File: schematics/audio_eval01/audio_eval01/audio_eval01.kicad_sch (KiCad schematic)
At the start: 21 parts, among them J1 Conn_01x10_Pin, J2 AudioJack3, J3 Conn_01x02_Pin, U2 AMS1117-1.8

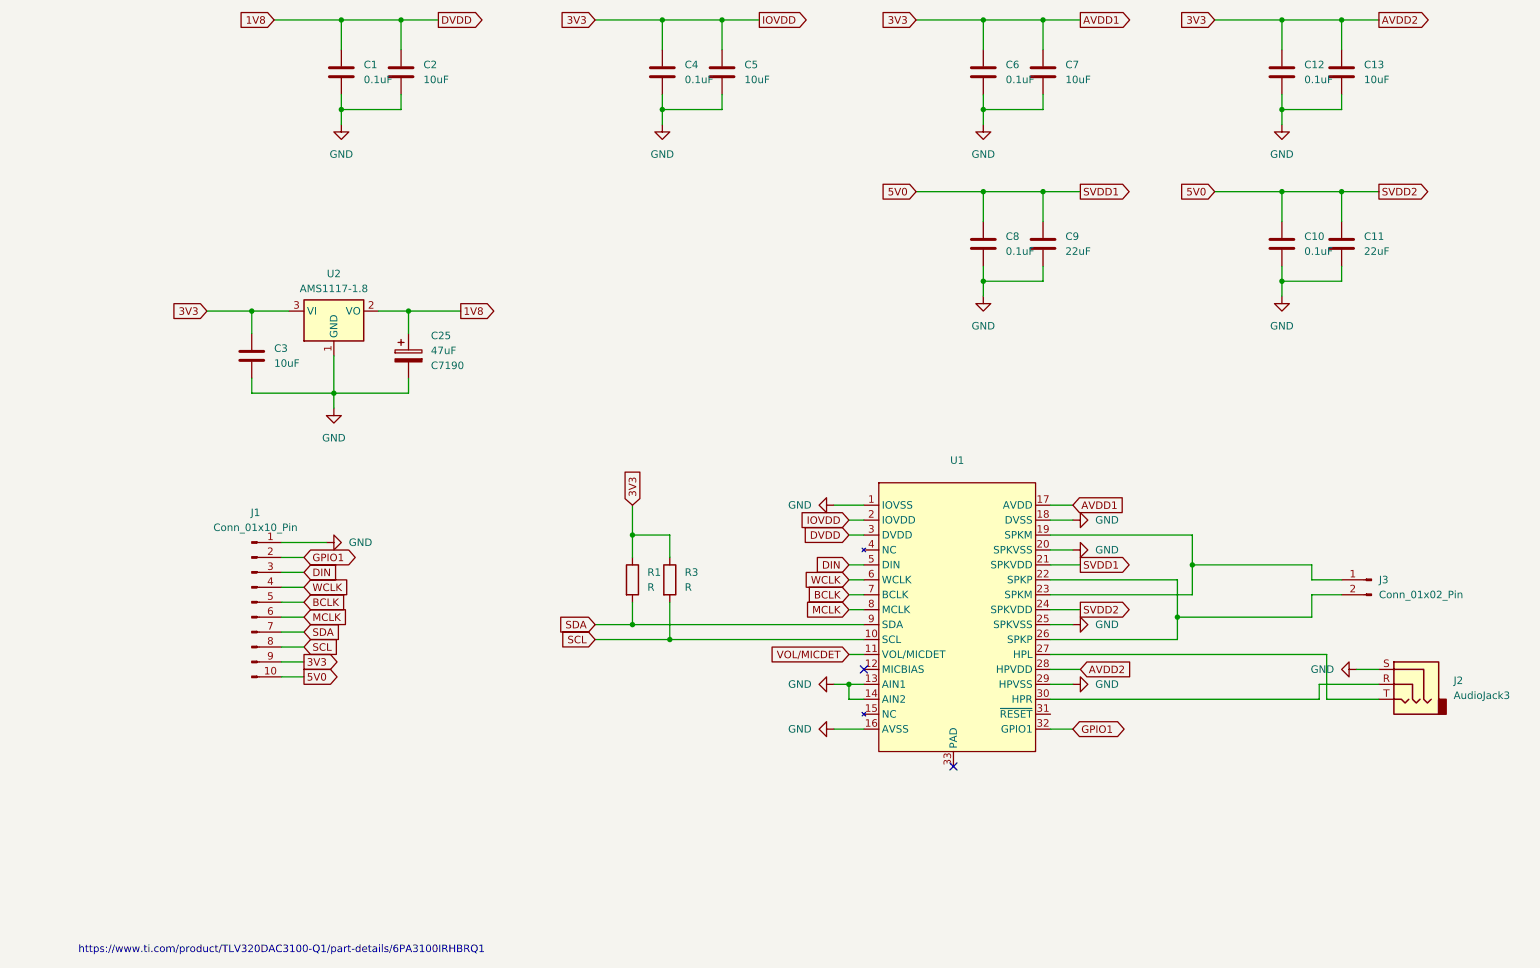
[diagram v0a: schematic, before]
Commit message: Prepared Audio evaluation board for manufacture.
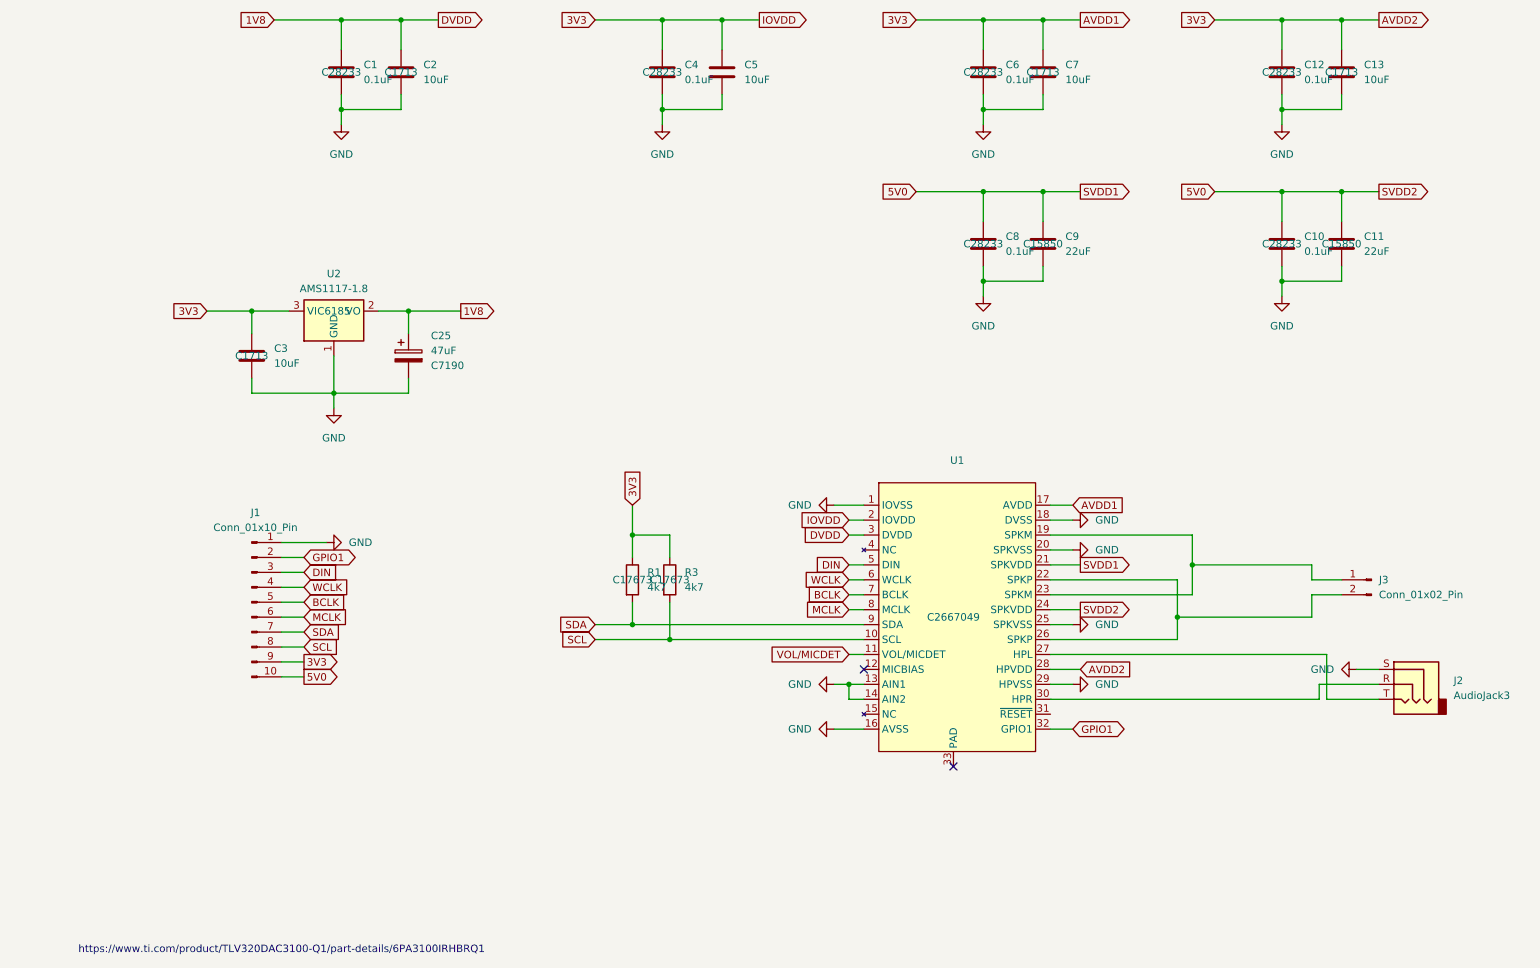
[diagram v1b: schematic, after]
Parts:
- C1, C10, C12, C4, C6, C8: LCSC (none) -> C28233
- C11, C9: LCSC (none) -> C15850
- C13, C2, C3, C5, C7: LCSC (none) -> C1713
- R1, R3: value R -> 4k7; LCSC (none) -> C17673
- U1: LCSC (none) -> C2667049
- U2: LCPC C6185 -> (none); LCSC (none) -> C6185
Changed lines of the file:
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@@
+			)
+		)
+		(property "LCSC" "C28233"
+			(at 226.06 68.58 0)
+			(effects
+				(font
+					(size 1.27 1.27)
+				)
 			)
 		)
@@
 			)
 		)
+		(property "LCSC" "C15850"
+			(at 236.22 68.58 0)
+			(effects
+				(font
+					(size 1.27 1.27)
+				)
+			)
+		)
 		(pin "2"
 		)
@@
 			)
 		)
+		(property "LCSC" "C1713"
+			(at 76.2 39.37 0)
+			(effects
+				(font
+					(size 1.27 1.27)
+				)
+			)
+		)
 		(pin "2"
 		)
@@
 			)
 		)
-		(property "Value" "R"
+		(property "Value" "4k7"
 			(at 124.46 126.9999 0)
 			(effects
@@
 			)
 		)
+		(property "LCSC" "C17673"
+			(at 121.92 125.73 0)
+			(effects
+				(font
+					(size 1.27 1.27)
+				)
+			)
+		)
 		(pin "2"
 		)
@@
 			)
 		)
+		(property "LCSC" "C28233"
+			(at 226.06 39.37 0)
+			(effects
+				(font
+					(size 1.27 1.27)
+				)
+			)
+		)
 		(pin "2"
 		)
@@
 			)
 		)
+		(property "LCSC" "C15850"
+			(at 185.42 68.58 0)
+			(effects
+				(font
+					(size 1.27 1.27)
+				)
+			)
+		)
 		(pin "2"
 		)
@@
 			)
 		)
+		(property "LCSC" "C1713"
+			(at 185.42 39.37 0)
+			(effects
+				(font
+					(size 1.27 1.27)
+				)
+			)
+		)
 		(pin "2"
 		)
@@
 			)
 		)
+		(property "LCSC" "C28233"
+			(at 120.65 39.37 0)
+			(effects
+				(font
+					(size 1.27 1.27)
+				)
+			)
+		)
 		(pin "2"
 		)
@@
 			)
 		)
+		(property "LCSC" "C28233"
+			(at 175.26 68.58 0)
+			(effects
+				(font
+					(size 1.27 1.27)
+				)
+			)
+		)
 		(pin "2"
 		)
@@
 			)
 		)
+		(property "LCSC" "C2667049"
+			(at 170.18 132.08 0)
+			(effects
+				(font
+					(size 1.27 1.27)
+				)
+			)
+		)
 		(pin "31"
 		)
@@
 			)
 		)
-		(property "Value" "R"
+		(property "Value" "4k7"
 			(at 118.11 126.9999 0)
 			(effects
@@
 				)
 				(hide yes)
+			)
+		)
+		(property "LCSC" "C17673"
+			(at 115.57 125.73 0)
+			(effects
+				(font
+					(size 1.27 1.27)
+				)
 			)
 		)
@@
 			)
 		)
+		(property "LCSC" "C1713"
+			(at 130.81 39.37 0)
+			(effects
+				(font
+					(size 1.27 1.27)
+				)
+				(hide yes)
+			)
+		)
 		(pin "2"
 		)
@@
 			)
 		)
+		(property "LCSC" "C1713"
+			(at 50.8 87.63 0)
+			(effects
+				(font
+					(size 1.27 1.27)
+				)
+			)
+		)
 		(pin "2"
 		)
@@
 			)
 		)
+		(property "LCSC" "C1713"
+			(at 236.22 39.37 0)
+			(effects
+				(font
+					(size 1.27 1.27)
+				)
+			)
+		)
 		(pin "2"
 		)
@@
 			)
 		)
+		(property "LCSC" "C28233"
+			(at 175.26 39.37 0)
+			(effects
+				(font
+					(size 1.27 1.27)
+				)
+			)
+		)
 		(pin "2"
 		)
@@
 			)
 		)
-		(property "LCPC" "C6185"
+		(property "LCSC" "C6185"
 			(at 64.77 80.01 0)
 			(effects
@@
 					(size 1.27 1.27)
 				)
-				(hide yes)
 			)
 		)
@@
 			)
 		)
+		(property "LCSC" "C28233"
+			(at 66.04 39.37 0)
+			(effects
+				(font
+					(size 1.27 1.27)
+				)
+			)
+		)
